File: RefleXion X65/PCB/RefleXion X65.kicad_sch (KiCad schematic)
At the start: 164 parts, among them SW1 SW_Push, SW10 SW_Push, SW11 SW_Push, SW12 SW_Push, SW13 SW_Push, SW14 SW_Push, SW15 SW_Push, SW16 SW_Push, SW17 SW_Push, SW18 SW_Push, SW19 SW_Push, SW2 SW_Push, SW20 SW_Push, SW21 SW_Push, SW22 SW_Push, SW23 SW_Push, SW24 SW_Push, SW25 SW_Push, SW26 SW_Push, SW27 SW_Push, SW28 SW_Push, SW29 SW_Push, SW3 SW_Push, SW30 SW_Push, SW31 SW_Push, SW32 SW_Push, SW33 SW_Push, SW34 SW_Push, SW35 SW_Push, SW36 SW_Push, SW4 SW_Push, SW5 SW_Push, SW6 SW_Push, SW7 SW_Push, SW8 SW_Push, SW9 SW_Push, U1 SN74LV1T34DBV, U2 SRV05-4, U5 SPX3819M5-L-3-3/TR, U6 SRV05-4, U7 W25Q32JVUUIQ, U8 RP2040, Y1 TXM12M0004252LBCEO00T

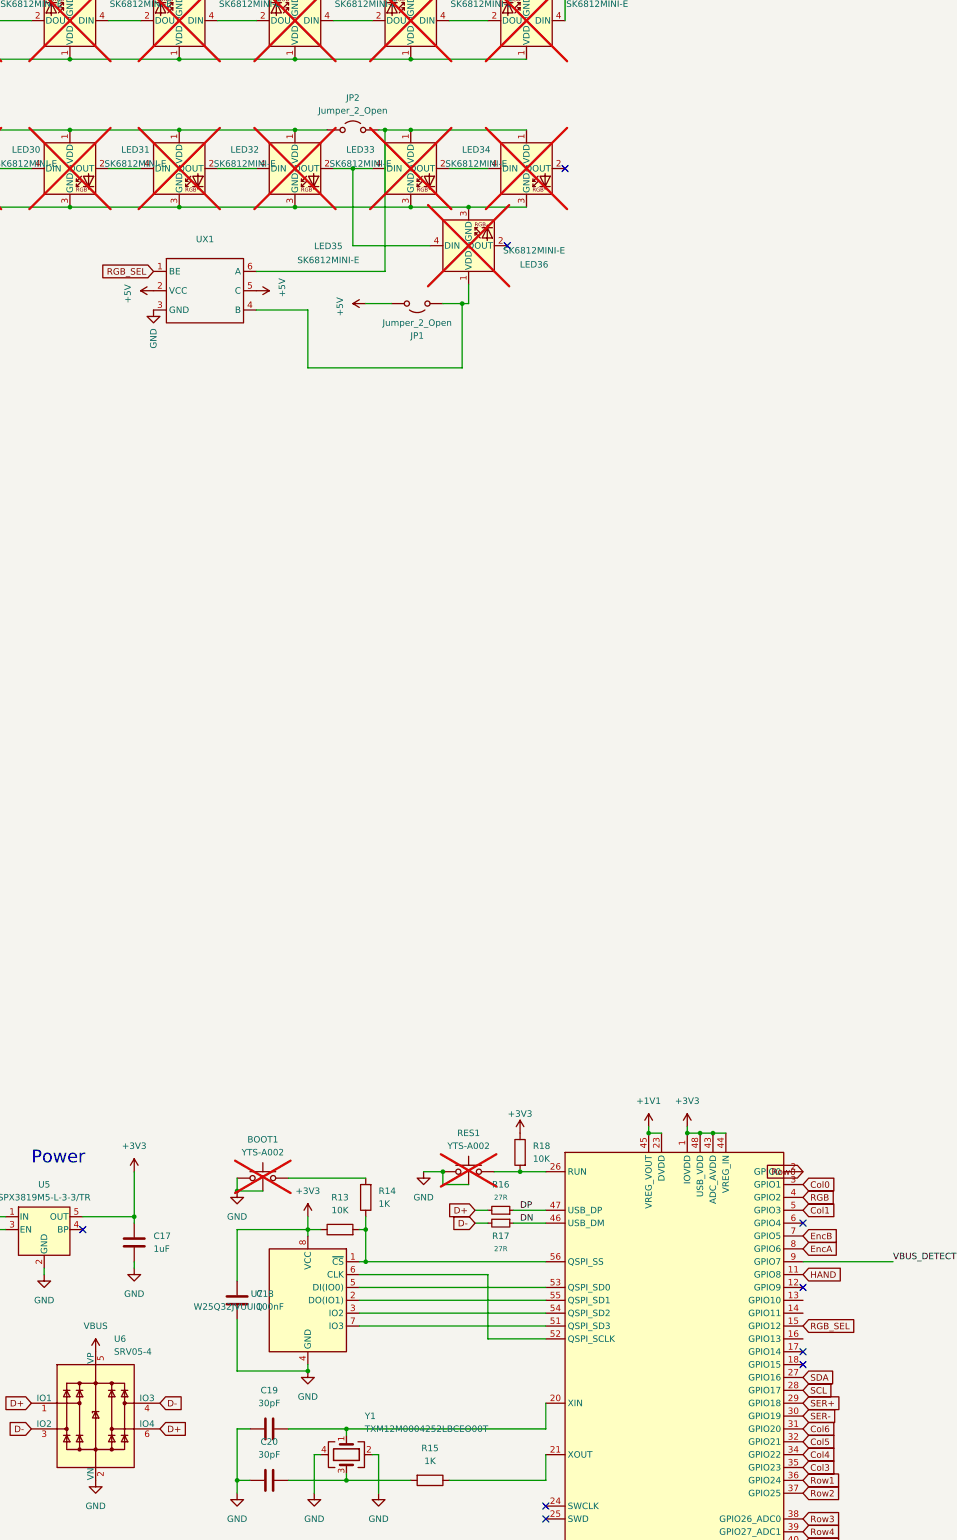
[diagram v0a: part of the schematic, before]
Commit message: Test Mosfet version
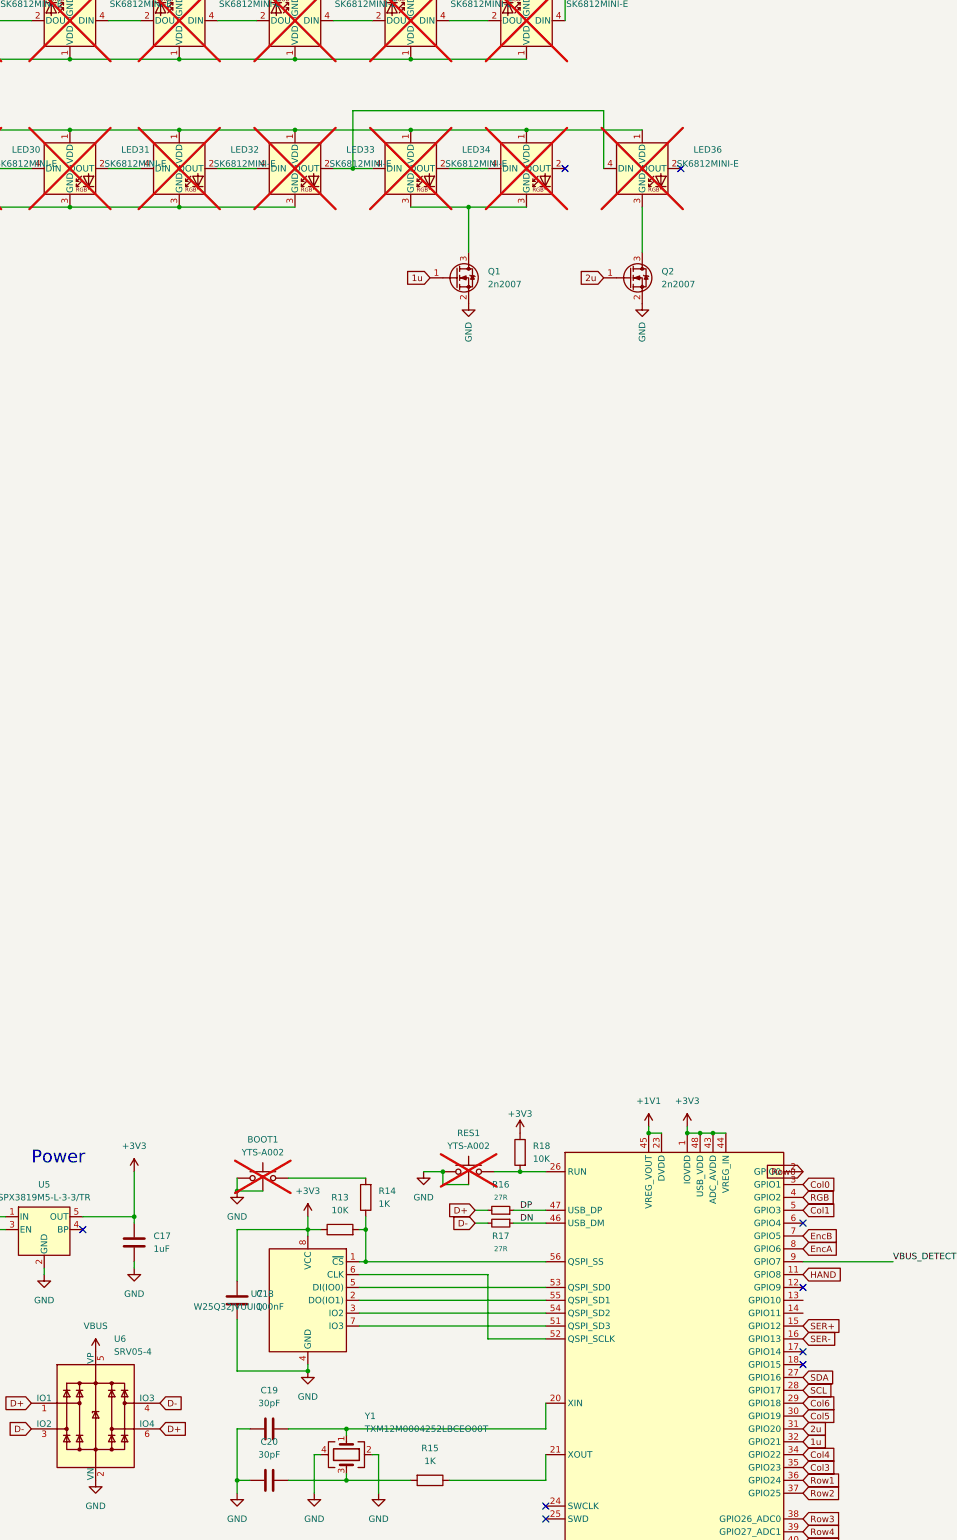
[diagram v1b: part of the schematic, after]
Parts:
- removed JP1, JP2: Jumper_2_Open, Keyboard Common:Jumper_min_v2, symbol Jumper:Jumper_2_Open
- removed UX1: ~, Package_TO_SOT_SMD:SOT-23-6, symbol Keyboard Common:PI5C3303
- added Q1, Q2: 2n2007, Package_TO_SOT_SMD:SOT-23, symbol Device:Q_NMOS_GSD
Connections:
- net RGB_SEL is gone; now on net SER+: U8.15 (GPIO12)
- net +5V: now also LED34.1 (VDD), LED35.1 (VDD), LED36.1 (VDD)
- net Col5: now also U8.30 (GPIO19); no longer U8.32 (GPIO21)
- net Col6: now also U8.29 (GPIO18); no longer U8.31 (GPIO20)
- net GND: now also Q1.2 (S), Q2.2 (S); no longer LED34.3 (GND), LED35.3 (GND), LED36.3 (GND)
- net SER+: no longer U8.29 (GPIO18)
- net SER-: now also U8.16 (GPIO13); no longer U8.30 (GPIO19)
- new net: LED34.3 (GND), LED35.3 (GND), Q1.3 (D)
- new net: LED36.3 (GND), Q2.3 (D)
- new net 1u: Q1.1 (G), U8.32 (GPIO21)
- new net 2u: Q2.1 (G), U8.31 (GPIO20)
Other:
- moved on the sheet: LED36

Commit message: Reflexion X65 v1.10
PCB finalized
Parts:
- added JP1, JP2: Jumper_2_Open, Keyboard Common:Jumper_min_v2, symbol Jumper:Jumper_2_Open
- added LED37, LED38, LED39, LED40, LED41, LED42, LED43, LED44: SK6812MINI-E, Keyboard RGB:MX_SK6812MINI-E_REVERSIBLE_special, symbol Keyboard Common:SK6812MINI-E
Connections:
- net +5V: now also JP1.1 (A), JP2.1 (A), LED37.1 (VDD), LED38.1 (VDD), LED39.1 (VDD), LED40.1 (VDD), LED41.1 (VDD), LED42.1 (VDD), LED43.1 (VDD), LED44.1 (VDD); no longer LED34.1 (VDD), LED35.1 (VDD), LED36.1 (VDD)
- net Col0: now also U8.38 (GPIO26_ADC0); no longer U8.3 (GPIO1)
- net Col1: now also U8.40 (GPIO28_ADC2); no longer U8.5 (GPIO3)
- net Col2: now also U8.36 (GPIO24); no longer U8.41 (GPIO29_ADC3)
- net Col3: now also U8.18 (GPIO15); no longer U8.35 (GPIO23)
- net Col4: now also U8.17 (GPIO14); no longer U8.34 (GPIO22)
- net Col5: now also U8.16 (GPIO13); no longer U8.30 (GPIO19)
- net Col6: now also U8.15 (GPIO12); no longer U8.29 (GPIO18)
- net EncA: now also U8.4 (GPIO2); no longer U8.8 (GPIO6)
- net EncB: now also U8.3 (GPIO1); no longer U8.7 (GPIO5)
- net GND: no longer LED1.3 (GND), LED10.3 (GND), LED11.3 (GND), LED12.3 (GND), LED13.3 (GND), LED14.3 (GND), LED15.3 (GND), LED16.3 (GND), LED17.3 (GND), LED18.3 (GND), LED19.3 (GND), LED2.3 (GND), LED20.3 (GND), LED21.3 (GND), LED22.3 (GND), LED23.3 (GND), LED24.3 (GND), LED25.3 (GND), LED26.3 (GND), LED27.3 (GND), LED28.3 (GND), LED29.3 (GND), LED3.3 (GND), LED30.3 (GND), LED31.3 (GND), LED32.3 (GND), LED33.3 (GND), LED4.3 (GND), LED5.3 (GND), LED6.3 (GND), LED7.3 (GND), LED8.3 (GND), LED9.3 (GND)
- net HAND: now also U8.14 (GPIO11); no longer U8.11 (GPIO8)
- net Row0: now also U8.41 (GPIO29_ADC3); no longer U8.2 (GPIO0)
- net Row1: now also U8.30 (GPIO19); no longer U8.36 (GPIO24)
- net Row2: now also U8.31 (GPIO20); no longer U8.37 (GPIO25)
- net Row3: now also U8.32 (GPIO21); no longer U8.38 (GPIO26_ADC0)
- net Row4: now also U8.34 (GPIO22); no longer U8.39 (GPIO27_ADC1)
- net Row5: now also U8.35 (GPIO23); no longer U8.40 (GPIO28_ADC2)
- net SCL: now also U8.7 (GPIO5); no longer U8.28 (GPIO17)
- net SDA: now also U8.6 (GPIO4); no longer U8.27 (GPIO16)
- net SER+: now also U8.12 (GPIO9); no longer U8.15 (GPIO12)
- net SER-: now also U8.13 (GPIO10); no longer U8.16 (GPIO13)
- net VBUS_DETECT: now also U8.39 (GPIO27_ADC1); no longer U8.9 (GPIO7)
- net RGB_5: now reaches LED1.4 (DIN), U1.4 (Y)
- net RGB_5: now also LED37.4 (DIN)
- net at LED34.3 (GND), LED35.3 (GND), Q1.3 (D): now also LED1.3 (GND), LED10.3 (GND), LED11.3 (GND), LED12.3 (GND), LED13.3 (GND), LED14.3 (GND), LED15.3 (GND), LED16.3 (GND), LED17.3 (GND), LED18.3 (GND), LED19.3 (GND), LED2.3 (GND), LED20.3 (GND), LED21.3 (GND), LED22.3 (GND), LED23.3 (GND), LED24.3 (GND), LED25.3 (GND), LED26.3 (GND), LED27.3 (GND), LED28.3 (GND), LED29.3 (GND), LED3.3 (GND), LED30.3 (GND), LED31.3 (GND), LED32.3 (GND), LED33.3 (GND), LED36.3 (GND), LED4.3 (GND), LED5.3 (GND), LED6.3 (GND), LED7.3 (GND), LED8.3 (GND), LED9.3 (GND)
- net at Q2.3 (D): now also LED37.3 (GND), LED38.3 (GND), LED39.3 (GND), LED40.3 (GND), LED41.3 (GND), LED42.3 (GND), LED43.3 (GND), LED44.3 (GND); no longer LED36.3 (GND)
- net 1u renamed KEY
- net KEY: now also U8.29 (GPIO18); no longer U8.32 (GPIO21)
- net 2u renamed GLOW
- net GLOW: now also U8.28 (GPIO17); no longer U8.31 (GPIO20)
- net RGB renamed RGB_3
- net RGB_3: now also U8.37 (GPIO25); no longer U8.4 (GPIO2)
- new net: LED43.2 (DOUT), LED44.4 (DIN)
- new net: JP2.2 (B), LED34.1 (VDD), LED35.1 (VDD)
- new net: LED37.2 (DOUT), LED38.4 (DIN)
- new net: LED41.2 (DOUT), LED42.4 (DIN)
- new net: LED40.2 (DOUT), LED41.4 (DIN)
- new net: LED42.2 (DOUT), LED43.4 (DIN)
- new net: LED39.2 (DOUT), LED40.4 (DIN)
- new net: LED38.2 (DOUT), LED39.4 (DIN)
- new net: JP1.2 (B), LED36.1 (VDD)
- no-connect marks 15 -> 18
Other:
- moved on the sheet: LED1, LED10, LED11, LED12, LED13, LED14, LED15, LED16, LED17, LED18, LED19, LED2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
